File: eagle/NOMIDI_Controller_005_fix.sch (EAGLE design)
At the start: 134 parts, among them IC1 4067D, IC2 4067D, IC3 4067D, IC4 4067D, IC5 4067D, M0 SLIDEPOT-ALPS-60MM, M1 SLIDEPOT-ALPS-60MM, P0_0 US-EVUF3A, P0_1 US-EVUF3A, P0_2 US-EVUF3A, P0_3 US-EVUF3A, P0_4 US-EVUF3A, P0_5 US-EVUF3A, P0_6 US-EVUF3A, P0_7 US-EVUF3A, P0_8 US-EVUF3A, P0_9 US-EVUF3A, P1_0 US-EVUF3A, P1_1 US-EVUF3A, P1_2 US-EVUF3A, P1_3 US-EVUF3A, P1_4 US-EVUF3A, P1_5 US-EVUF3A, P1_6 US-EVUF3A, P1_7 US-EVUF3A, P1_8 US-EVUF3A, P1_9 US-EVUF3A, T1 BC547, T10 BC547, T2 BC547, T3 BC547, T4 BC547, T5 BC547, T6 BC547, T7 BC547, T8 BC547, T9 BC547

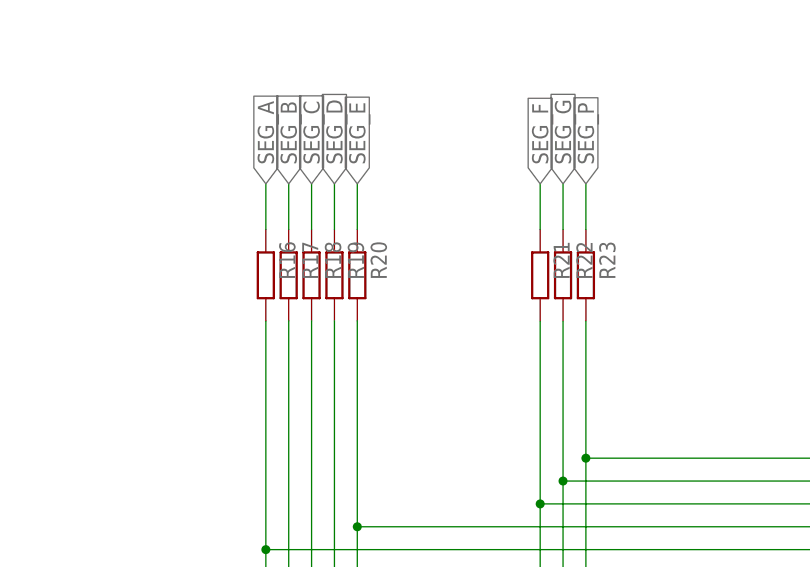
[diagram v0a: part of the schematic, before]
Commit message: bom link
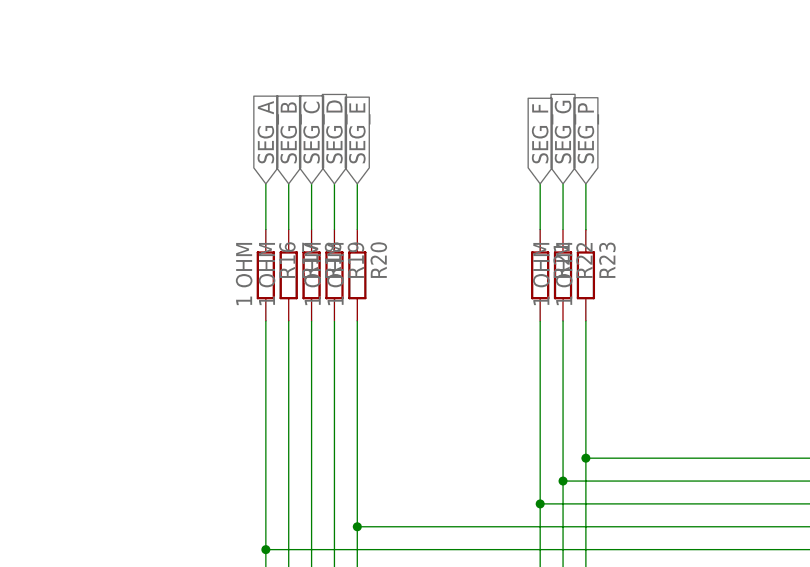
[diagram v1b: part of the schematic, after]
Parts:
- R16, R17, R19, R20, R22, R23: value (none) -> 1 OHM
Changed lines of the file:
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@@
 <part name="R14" library="rcl" library_urn="urn:adsk.eagle:library:334" deviceset="R-EU_" device="0207/7" package3d_urn="urn:adsk.eagle:package:23493/2" value="4k7"/>
 <part name="R15" library="rcl" library_urn="urn:adsk.eagle:library:334" deviceset="R-EU_" device="0207/7" package3d_urn="urn:adsk.eagle:package:23493/2" value="4k7"/>
-<part name="R16" library="rcl" library_urn="urn:adsk.eagle:library:334" deviceset="R-EU_" device="0207/7" package3d_urn="urn:adsk.eagle:package:23493/2"/>
-<part name="R17" library="rcl" library_urn="urn:adsk.eagle:library:334" deviceset="R-EU_" device="0207/7" package3d_urn="urn:adsk.eagle:package:23493/2"/>
+<part name="R16" library="rcl" library_urn="urn:adsk.eagle:library:334" deviceset="R-EU_" device="0207/7" package3d_urn="urn:adsk.eagle:package:23493/2" value="1 OHM"/>
+<part name="R17" library="rcl" library_urn="urn:adsk.eagle:library:334" deviceset="R-EU_" device="0207/7" package3d_urn="urn:adsk.eagle:package:23493/2" value="1 OHM"/>
 <part name="R18" library="rcl" library_urn="urn:adsk.eagle:library:334" deviceset="R-EU_" device="0207/7" package3d_urn="urn:adsk.eagle:package:23493/2"/>
-<part name="R19" library="rcl" library_urn="urn:adsk.eagle:library:334" deviceset="R-EU_" device="0207/7" package3d_urn="urn:adsk.eagle:package:23493/2"/>
-<part name="R20" library="rcl" library_urn="urn:adsk.eagle:library:334" deviceset="R-EU_" device="0207/7" package3d_urn="urn:adsk.eagle:package:23493/2"/>
+<part name="R19" library="rcl" library_urn="urn:adsk.eagle:library:334" deviceset="R-EU_" device="0207/7" package3d_urn="urn:adsk.eagle:package:23493/2" value="1 OHM"/>
+<part name="R20" library="rcl" library_urn="urn:adsk.eagle:library:334" deviceset="R-EU_" device="0207/7" package3d_urn="urn:adsk.eagle:package:23493/2" value="1 OHM"/>
 <part name="R21" library="rcl" library_urn="urn:adsk.eagle:library:334" deviceset="R-EU_" device="0207/7" package3d_urn="urn:adsk.eagle:package:23493/2"/>
-<part name="R22" library="rcl" library_urn="urn:adsk.eagle:library:334" deviceset="R-EU_" device="0207/7" package3d_urn="urn:adsk.eagle:package:23493/2"/>
-<part name="R23" library="rcl" library_urn="urn:adsk.eagle:library:334" deviceset="R-EU_" device="0207/7" package3d_urn="urn:adsk.eagle:package:23493/2"/>
+<part name="R22" library="rcl" library_urn="urn:adsk.eagle:library:334" deviceset="R-EU_" device="0207/7" package3d_urn="urn:adsk.eagle:package:23493/2" value="1 OHM"/>
+<part name="R23" library="rcl" library_urn="urn:adsk.eagle:library:334" deviceset="R-EU_" device="0207/7" package3d_urn="urn:adsk.eagle:package:23493/2" value="1 OHM"/>
 <part name="D5" library="special" library_urn="urn:adsk.eagle:library:367" deviceset="7SEG-CK" device="" package3d_urn="urn:adsk.eagle:package:26668/2"/>
 <part name="D6" library="special" library_urn="urn:adsk.eagle:library:367" deviceset="7SEG-CK" device="" package3d_urn="urn:adsk.eagle:package:26668/2"/>
